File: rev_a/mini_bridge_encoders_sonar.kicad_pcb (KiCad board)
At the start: 2 copper layers, 4 parts

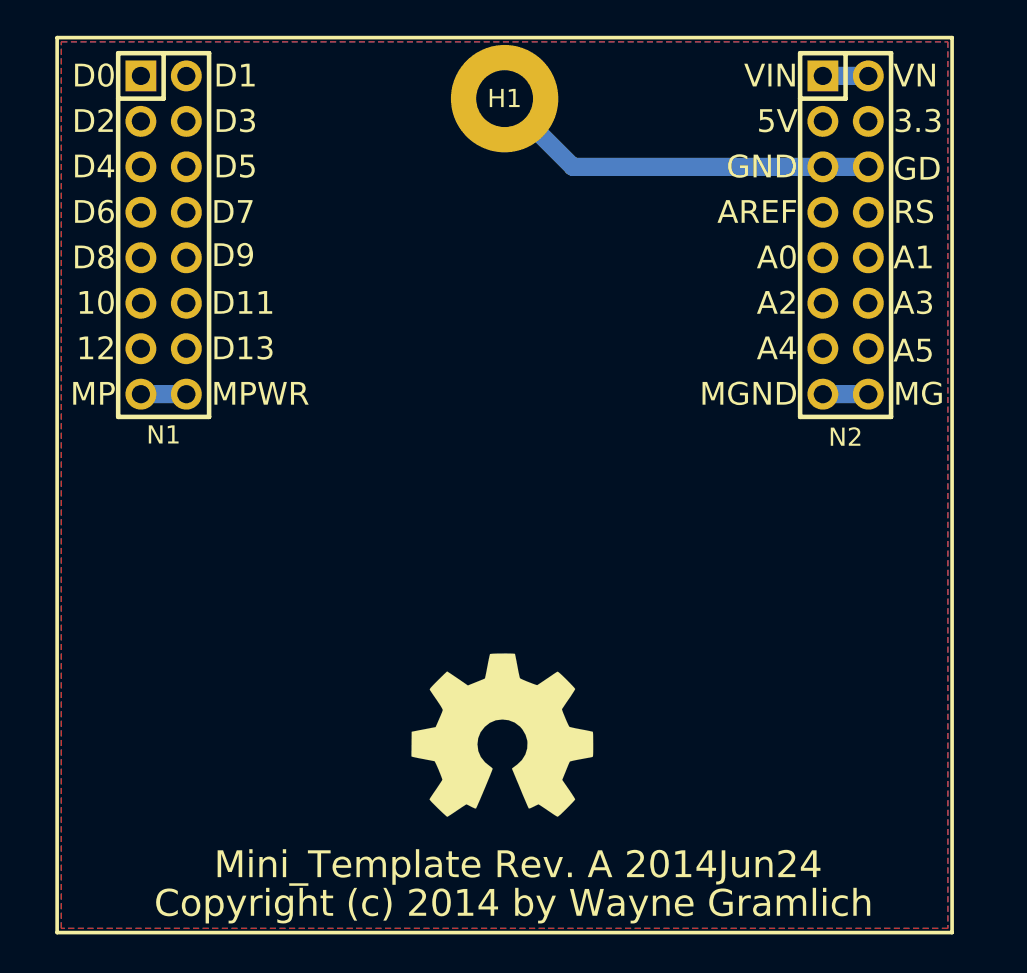
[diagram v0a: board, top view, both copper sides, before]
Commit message: Initial layout is complete.
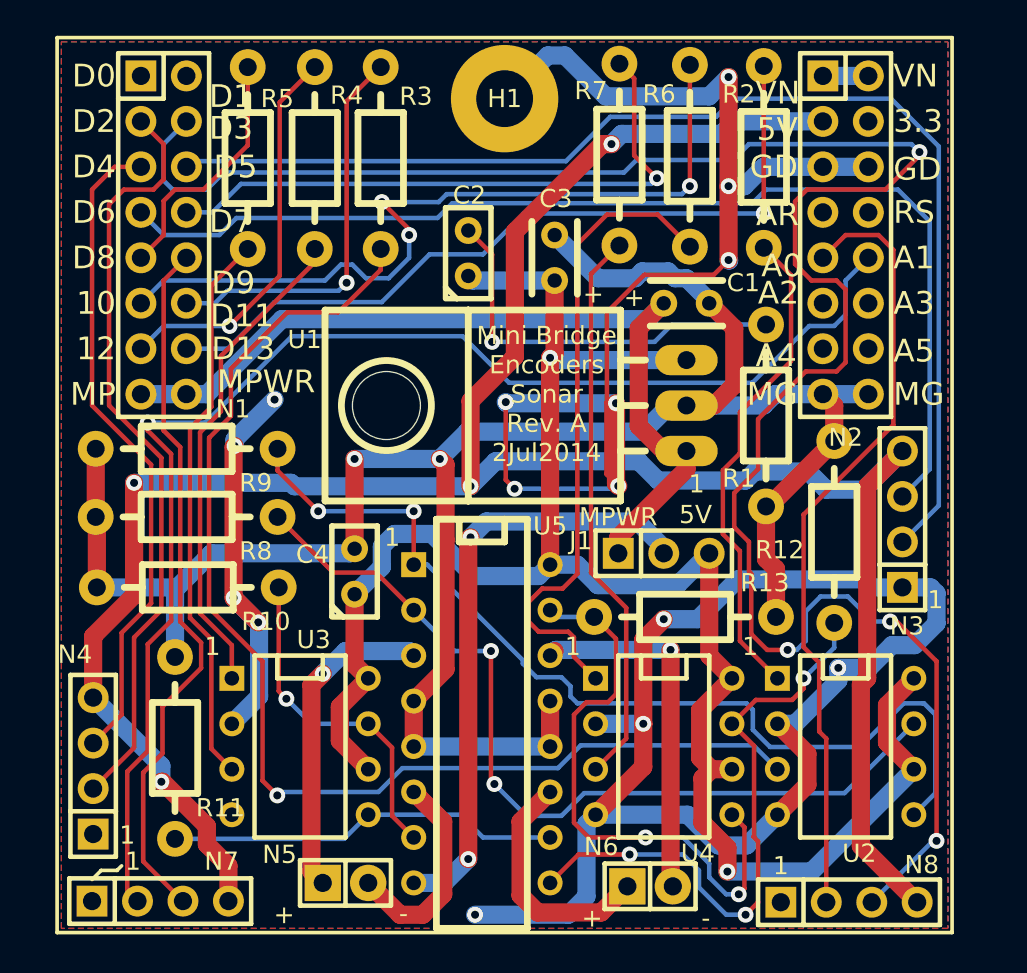
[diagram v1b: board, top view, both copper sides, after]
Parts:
- added C1: 22uF, Mini_Bridge_Encoders_Sonar_Rev_A:Capacitor4x3RM2-5_RevB, F.Cu at (111.8, 118.1)
- added C2: .1uF, Mini_Bridge_Encoders_Sonar_Rev_A:Capacitor3MMDiscRM2.5, F.Cu at (99.6, 115.3)
- added C3: 22uF, Mini_Bridge_Encoders_Sonar_Rev_A:Capacitor4x3RM2-5_RevB, F.Cu at (104.4, 115.6)
- added C4: .1uF, Mini_Bridge_Encoders_Sonar_Rev_A:Capacitor3MMDiscRM2.5, F.Cu at (93.2, 133.1)
- added J1: POWER_SELECT, Mini_Bridge_Encoders_Sonar_Rev_A:Pin_Header_Straight_1x03, F.Cu at (110.5, 132.1)
- added N3: ENCODER_CONNECTOR, Mini_Bridge_Encoders_Sonar_Rev_A:Pin_Header_Straight_1x04, F.Cu at (123.8, 130.2)
- added N4: ENCODER_CONNECTOR, Mini_Bridge_Encoders_Sonar_Rev_A:Pin_Header_Straight_1x04, F.Cu at (78.6, 144.0)
- added N5: MOTOR_CONNECTOR, Mini_Bridge_Encoders_Sonar_Rev_A:Pin_Header_Straight_1x02, F.Cu at (92.7, 150.5)
- added N6: MOTOR_CONNECTOR, Mini_Bridge_Encoders_Sonar_Rev_A:Pin_Header_Straight_1x02, F.Cu at (109.7, 150.7)
- added N7: HC_SR04_CONNECTOR, Mini_Bridge_Encoders_Sonar_Rev_A:Pin_Header_Straight_1x04, F.Cu at (82.4, 151.5)
- added N8: HC_SR04_CONNECTOR, Mini_Bridge_Encoders_Sonar_Rev_A:Pin_Header_Straight_1x04, F.Cu at (120.8, 151.6)
- added R1: .47, Mini_Bridge_Encoders_Sonar_Rev_A:Resistor_Horizontal_RM10mm, F.Cu at (116.2, 124.5)
- added R10: 10K, Mini_Bridge_Encoders_Sonar_Rev_A:Resistor_Horizontal_RM10mm, F.Cu at (83.8, 134.0)
- added R11: 10K, Mini_Bridge_Encoders_Sonar_Rev_A:Resistor_Horizontal_RM10mm, F.Cu at (83.2, 142.9)
- added R12: 10K, Mini_Bridge_Encoders_Sonar_Rev_A:Resistor_Horizontal_RM10mm, F.Cu at (120.0, 130.8)
- added R13: 10K, Mini_Bridge_Encoders_Sonar_Rev_A:Resistor_Horizontal_RM10mm, F.Cu at (111.8, 135.6)
- added R2: 470, Mini_Bridge_Encoders_Sonar_Rev_A:Resistor_Horizontal_RM10mm, F.Cu at (116.1, 109.9)
- added R3: 470, Mini_Bridge_Encoders_Sonar_Rev_A:Resistor_Horizontal_RM10mm, F.Cu at (94.7, 109.9)
- added R4: 470, Mini_Bridge_Encoders_Sonar_Rev_A:Resistor_Horizontal_RM10mm, F.Cu at (91.0, 109.9)
- added R5: 470, Mini_Bridge_Encoders_Sonar_Rev_A:Resistor_Horizontal_RM10mm, F.Cu at (87.2, 109.9)
- added R6: 470, Mini_Bridge_Encoders_Sonar_Rev_A:Resistor_Horizontal_RM10mm, F.Cu at (112.0, 109.8)
- added R7: 470, Mini_Bridge_Encoders_Sonar_Rev_A:Resistor_Horizontal_RM10mm, F.Cu at (108.0, 109.7)
- added R8: 10K, Mini_Bridge_Encoders_Sonar_Rev_A:Resistor_Horizontal_RM10mm, F.Cu at (83.8, 130.0)
- added R9: 10K, Mini_Bridge_Encoders_Sonar_Rev_A:Resistor_Horizontal_RM10mm, F.Cu at (83.8, 126.2)
- added U1: LM2940, Mini_Bridge_Encoders_Sonar_Rev_A:TO-220_Neutral123_Horizontal_LargePads, F.Cu at (111.8, 123.8)
- added U2: LTV-826, Mini_Bridge_Encoders_Sonar_Rev_A:DIP-8__300, F.Cu at (120.7, 142.9)
- added U3: LTV-826, Mini_Bridge_Encoders_Sonar_Rev_A:DIP-8__300, F.Cu at (90.2, 142.9)
- added U4: LTV-826, Mini_Bridge_Encoders_Sonar_Rev_A:DIP-8__300, F.Cu at (110.5, 142.9)
- added U5: 754410, Mini_Bridge_Encoders_Sonar_Rev_A:DIP-16__300, F.Cu at (100.3, 141.6)
- G1: moved to B.Cu
- moved G1 19.1 mm to (104.0, 123.3)
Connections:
- net /GND renamed GND
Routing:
- net GND: track 21.9 -> 175.5 mm, vias 0 -> 15
- net /5V: track 0.00 -> 135.5 mm, vias 0 -> 4
- net /MGND: track 2.54 -> 123.0 mm, vias 0 -> 2
- net /D3: track 0.00 -> 115.3 mm, vias 0 -> 4
- net /M5V: track 0.00 -> 105.0 mm, vias 0 -> 2
- net /A1: track 0.00 -> 75.9 mm, vias 0 -> 1
- net /D5: track 0.00 -> 68.3 mm
- net Net-(R3-Pad2): track 0.00 -> 67.4 mm, vias 0 -> 1
- net /D6: track 0.00 -> 62.4 mm
- net Net-(R9-Pad2): track 0.00 -> 54.6 mm, vias 0 -> 2
- net /MPWR: track 2.54 -> 51.6 mm
- net Net-(R8-Pad2): track 0.00 -> 48.8 mm, vias 0 -> 2
- net /D10: track 0.00 -> 44.8 mm, vias 0 -> 3
- net /A0: track 0.00 -> 43.9 mm
- net /D13: track 0.00 -> 43.6 mm, vias 0 -> 1
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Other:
- board text added: "+"
- board text added: "-"
- board text added: "1"
- board text added: "AR"
- board text added: "Copyright (c) 2014 Wayne Gramlich"
- board text added: "Mini Bridge Encoders Sonar"
- board text added: "Mini Bridge Encoders Sonar Rev. A 2Jul2014"
- board text added: "Open"
- board text added: "Rev. A 24Jul2014"
- board text added: "hardware"
- board text removed: "AREF"
- board text removed: "Copyright (c) 2014 by Wayne Gramlich"
- board text removed: "GND"
- board text removed: "MGND"
- board text removed: "Mini_Template Rev. A 2014Jun24"
- board text removed: "VIN"
